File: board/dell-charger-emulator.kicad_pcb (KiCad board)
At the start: 2 copper layers, 20.8 x 8.1 mm, 6 parts, among them J1 CONN_01X03, J2 CONN_01X02, U1 ATTINY85-20SU, U2 MC78L05ACD

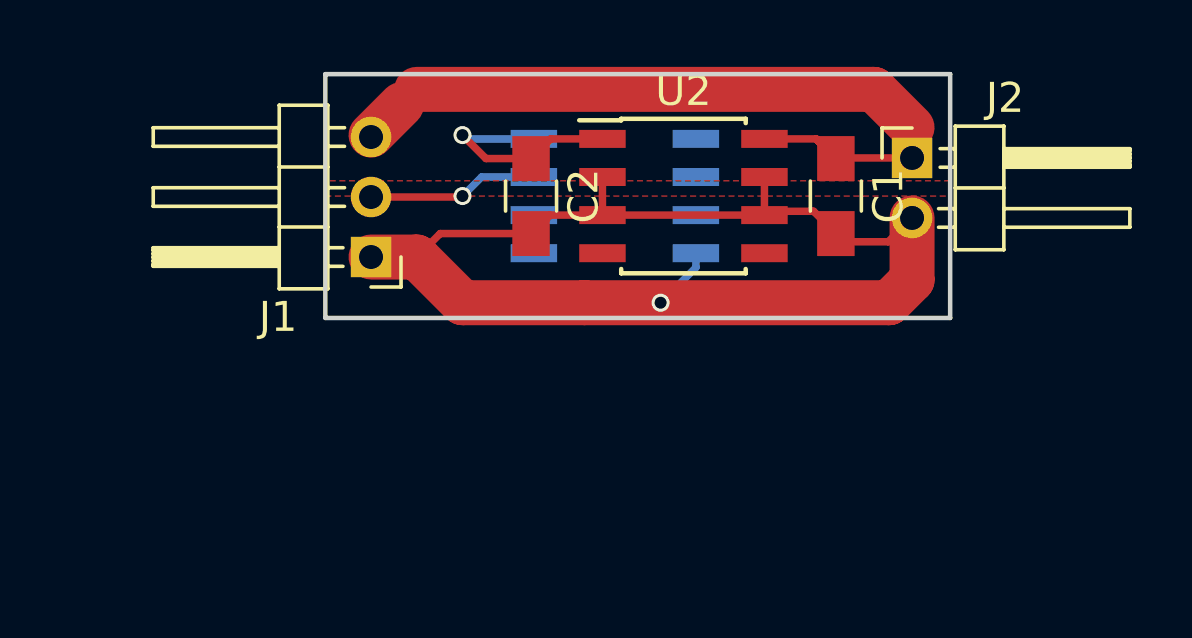
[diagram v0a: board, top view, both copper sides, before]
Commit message: Update board
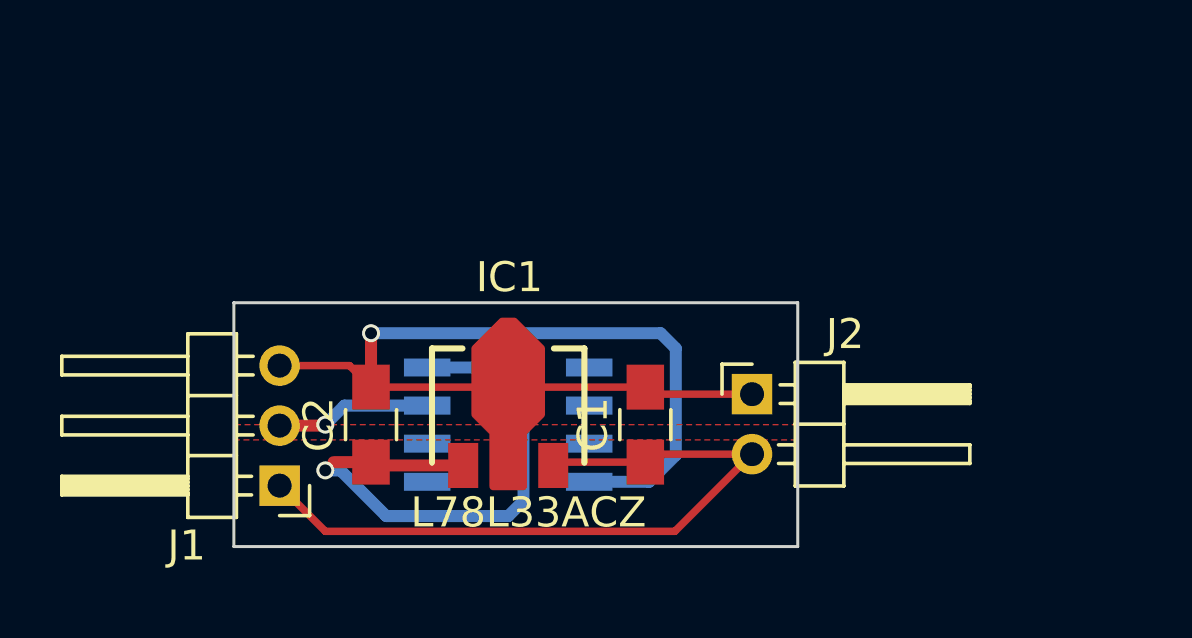
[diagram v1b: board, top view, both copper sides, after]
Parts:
- removed U2: MC78L05ACD, Housings_SOIC:SOIC-8_3.9x4.9mm_Pitch1.27mm
- added IC1: L78L33ACZ, SOT-89-3:SOT-89-3, F.Cu at (152.9, 109.2)
- moved C1 9.92 mm to (157.5, 111.8), turned to 90 degrees
- moved J2 9.51 mm to (161.0, 110.7)
- moved C2 9.30 mm to (148.3, 111.8), turned to 90 degrees
- moved U1 8.41 mm to (152.9, 111.8)
- moved J1 8.21 mm to (145.3, 113.8)
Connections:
- J1 pad 1: GND -> VCC
- J1 pad 3: VCC -> GND
- J2 pad 1: VCC -> GND
- J2 pad 2: GND -> VCC
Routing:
- net +3V3: track 7.69 -> 19.3 mm
- net GND: track 47.7 -> 37.6 mm
- net VCC: track 27.8 -> 24.2 mm
- net Net-(J1-Pad2): track 5.70 -> 5.20 mm
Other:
- board size 20.8 x 8.1 mm -> 18.8 x 8.1 mm
- net class Default: clearance 0.2 -> 0.25; trace_width 0.25 -> 0.4
- net class Power removed
- rule pad_to_mask_clearance: 0.2 -> 0
- rule trace_clearance: 0.2 -> 0.25
